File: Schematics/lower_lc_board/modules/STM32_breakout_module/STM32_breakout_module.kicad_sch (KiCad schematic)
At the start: 55 parts, among them J2 SWD_CONN, J3 USB_C_CONN, Q4 2N7002, SW1 SW_STM_RESET, SW2 SW_STM_BOOT_MODE, U5 STM32F103CBT6, U6 W25Q128JVS, U7 ISO1044BDR, U8 CP2102N-Axx-xQFN20, Y1 X322516MMB4SI

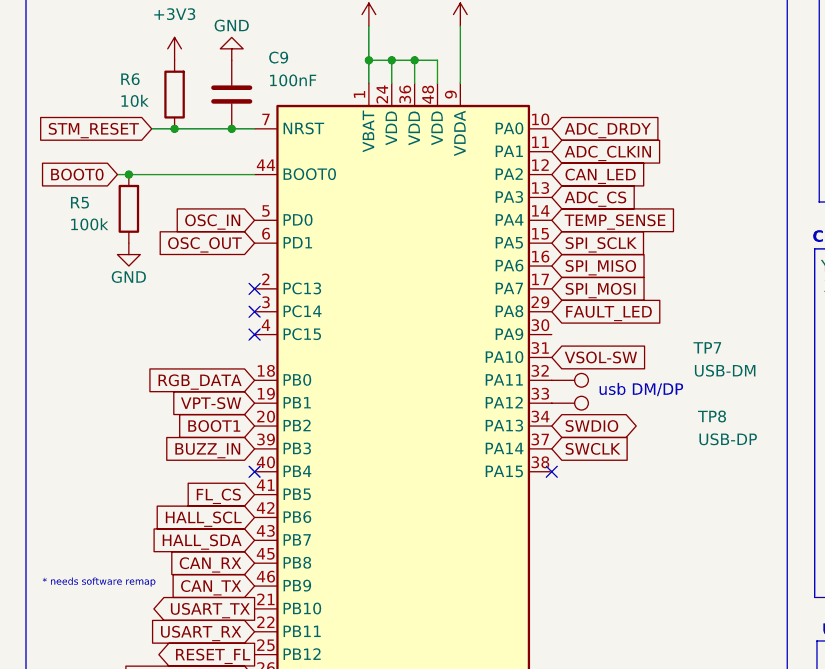
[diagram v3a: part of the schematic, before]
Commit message: more routing work
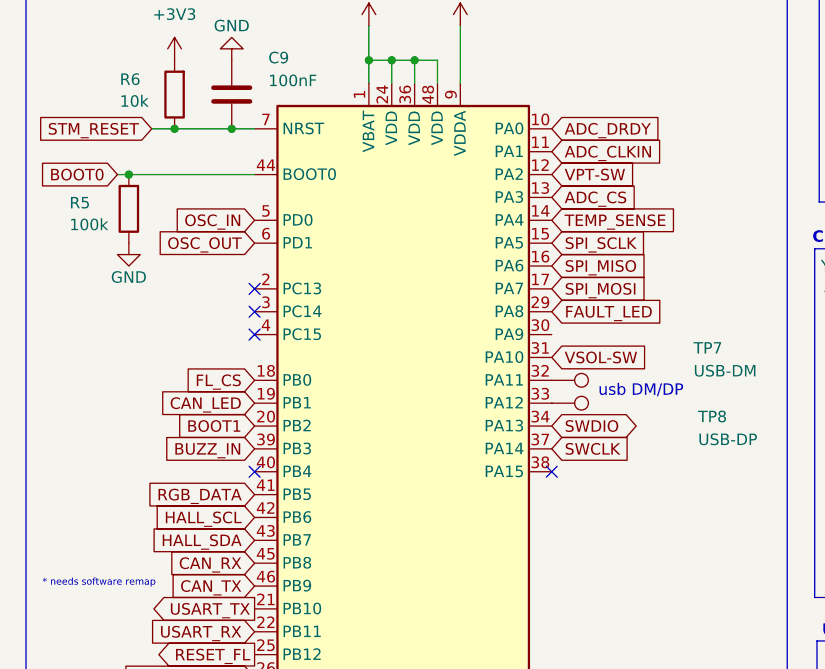
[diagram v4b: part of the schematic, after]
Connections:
- net CAN_LED: now also U5.19 (PB1); no longer U5.12 (PA2)
- net FL_CS: now also U5.18 (PB0); no longer U5.41 (PB5)
- net RGB_DATA: now also U5.41 (PB5); no longer U5.18 (PB0)
- net VPT-SW: now also U5.12 (PA2); no longer U5.19 (PB1)
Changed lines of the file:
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@@
-		)
-	)
-	(global_label "CAN_LED"
-		(shape input)
-		(at 74.93 53.34 0)
-		(fields_autoplaced yes)
-		(effects
-			(font
-				(size 1.27 1.27)
-			)
-			(justify left)
-		)
-		(property "Intersheetrefs" "${INTERSHEET_REFS}"
-			(at 86.019 53.34 0)
-			(effects
-				(font
-					(size 1.27 1.27)
-				)
-				(justify left)
-				(hide yes)
-			)
 		)
 	)
@@
 		)
 	)
-	(global_label "RGB_DATA"
+	(global_label "FL_CS"
 		(shape input)
 		(at 41.91 76.2 180)
@@
 		)
 		(property "Intersheetrefs" "${INTERSHEET_REFS}"
-			(at 29.7324 76.2 0)
+			(at 33.361 76.2 0)
 			(effects
 				(font
@@
 		)
 	)
+	(global_label "CAN_LED"
+		(shape input)
+		(at 41.91 78.74 180)
+		(fields_autoplaced yes)
+		(effects
+			(font
+				(size 1.27 1.27)
+			)
+			(justify right)
+		)
+		(property "Intersheetrefs" "${INTERSHEET_REFS}"
+			(at 30.821 78.74 0)
+			(effects
+				(font
+					(size 1.27 1.27)
+				)
+				(justify right)
+				(hide yes)
+			)
+		)
+	)
 	(global_label "OSC_IN"
 		(shape input)
@@
 		(property "Intersheetrefs" "${INTERSHEET_REFS}"
 			(at 157.5186 87.63 0)
-			(effects
-				(font
-					(size 1.27 1.27)
-				)
-				(justify right)
-				(hide yes)
-			)
-		)
-	)
-	(global_label "VPT-SW"
-		(shape input)
-		(at 41.91 78.74 180)
-		(fields_autoplaced yes)
-		(effects
-			(font
-				(size 1.27 1.27)
-			)
-			(justify right)
-		)
-		(property "Intersheetrefs" "${INTERSHEET_REFS}"
-			(at 31.3653 78.74 0)
 			(effects
 				(font
@@
 		)
 	)
+	(global_label "VPT-SW"
+		(shape input)
+		(at 74.93 53.34 0)
+		(fields_autoplaced yes)
+		(effects
+			(font
+				(size 1.27 1.27)
+			)
+			(justify left)
+		)
+		(property "Intersheetrefs" "${INTERSHEET_REFS}"
+			(at 85.4747 53.34 0)
+			(effects
+				(font
+					(size 1.27 1.27)
+				)
+				(justify left)
+				(hide yes)
+			)
+		)
+	)
 	(global_label "SWDIO"
 		(shape input)
@@
 		)
 	)
+	(global_label "RGB_DATA"
+		(shape input)
+		(at 41.91 88.9 180)
+		(fields_autoplaced yes)
+		(effects
+			(font
+				(size 1.27 1.27)
+			)
+			(justify right)
+		)
+		(property "Intersheetrefs" "${INTERSHEET_REFS}"
+			(at 29.7324 88.9 0)
+			(effects
+				(font
+					(size 1.27 1.27)
+				)
+				(justify right)
+				(hide yes)
+			)
+		)
+	)
 	(global_label "USB_N"
 		(shape input)
@@
 			(effects
 				(font
-					(size 1.27 1.27)
-				)
-				(justify right)
-				(hide yes)
-			)
-		)
-	)
-	(global_label "FL_CS"
-		(shape input)
-		(at 41.91 88.9 180)
-		(fields_autoplaced yes)
-		(effects
-			(font
-				(size 1.27 1.27)
-			)
-			(justify right)
-		)
-		(property "Intersheetrefs" "${INTERSHEET_REFS}"
-			(at 33.361 88.9 0)
-			(effects
-				(font
